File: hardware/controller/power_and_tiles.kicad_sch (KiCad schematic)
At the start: 27 parts, among them U1 XDJK-0051-025, U2 EA8212HT6R, U3 MT3406

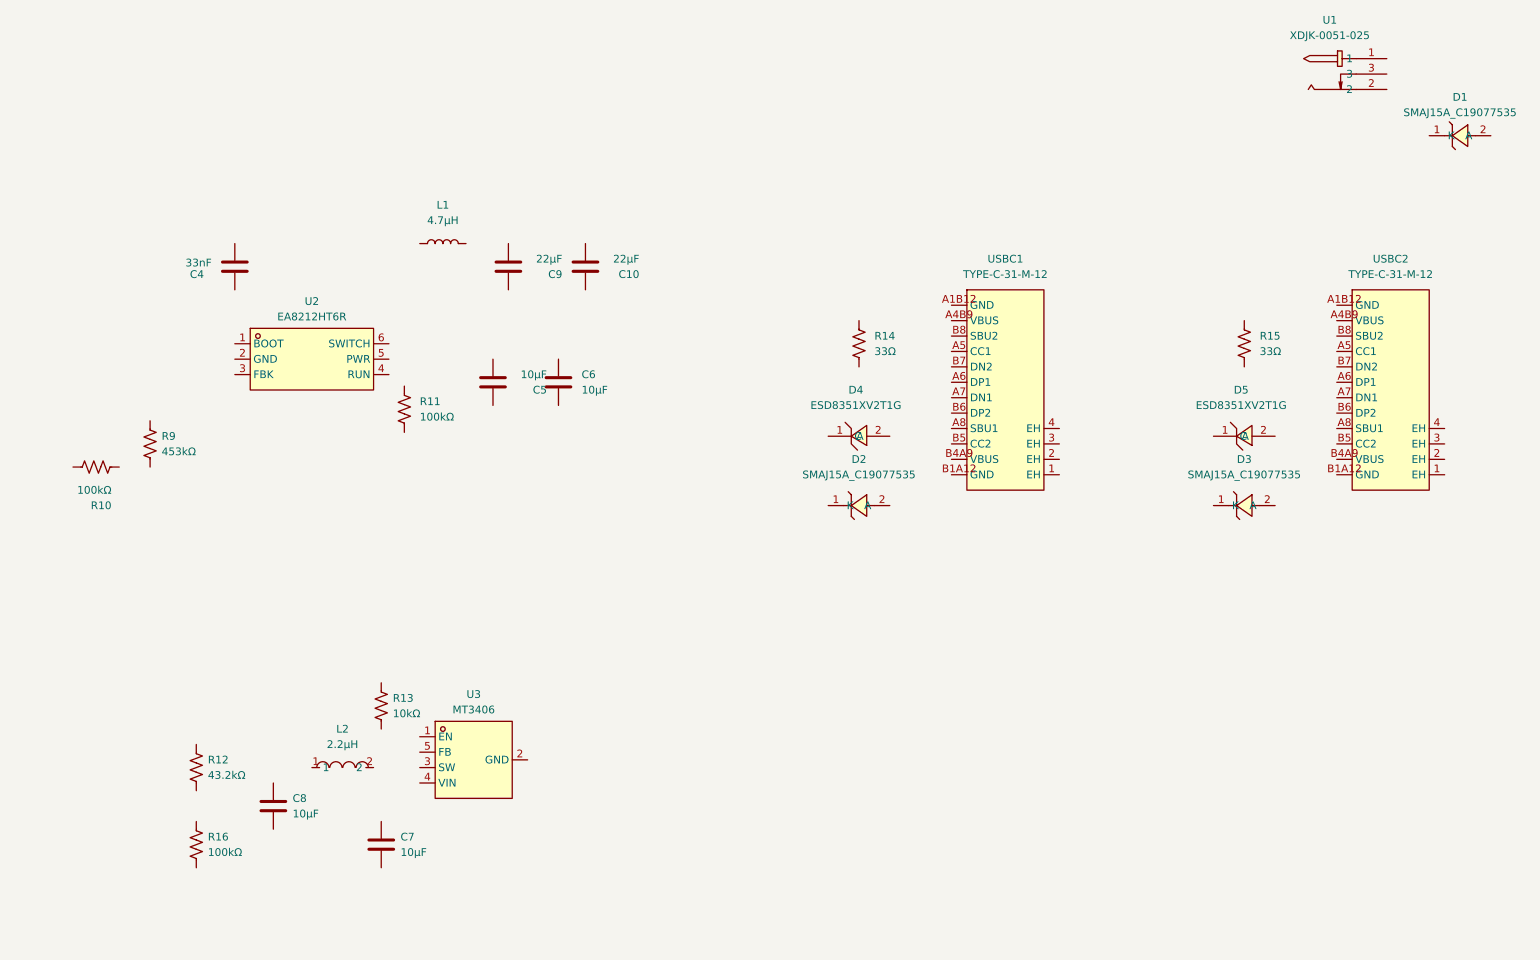
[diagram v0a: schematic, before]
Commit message: hooking up parts in the schematic
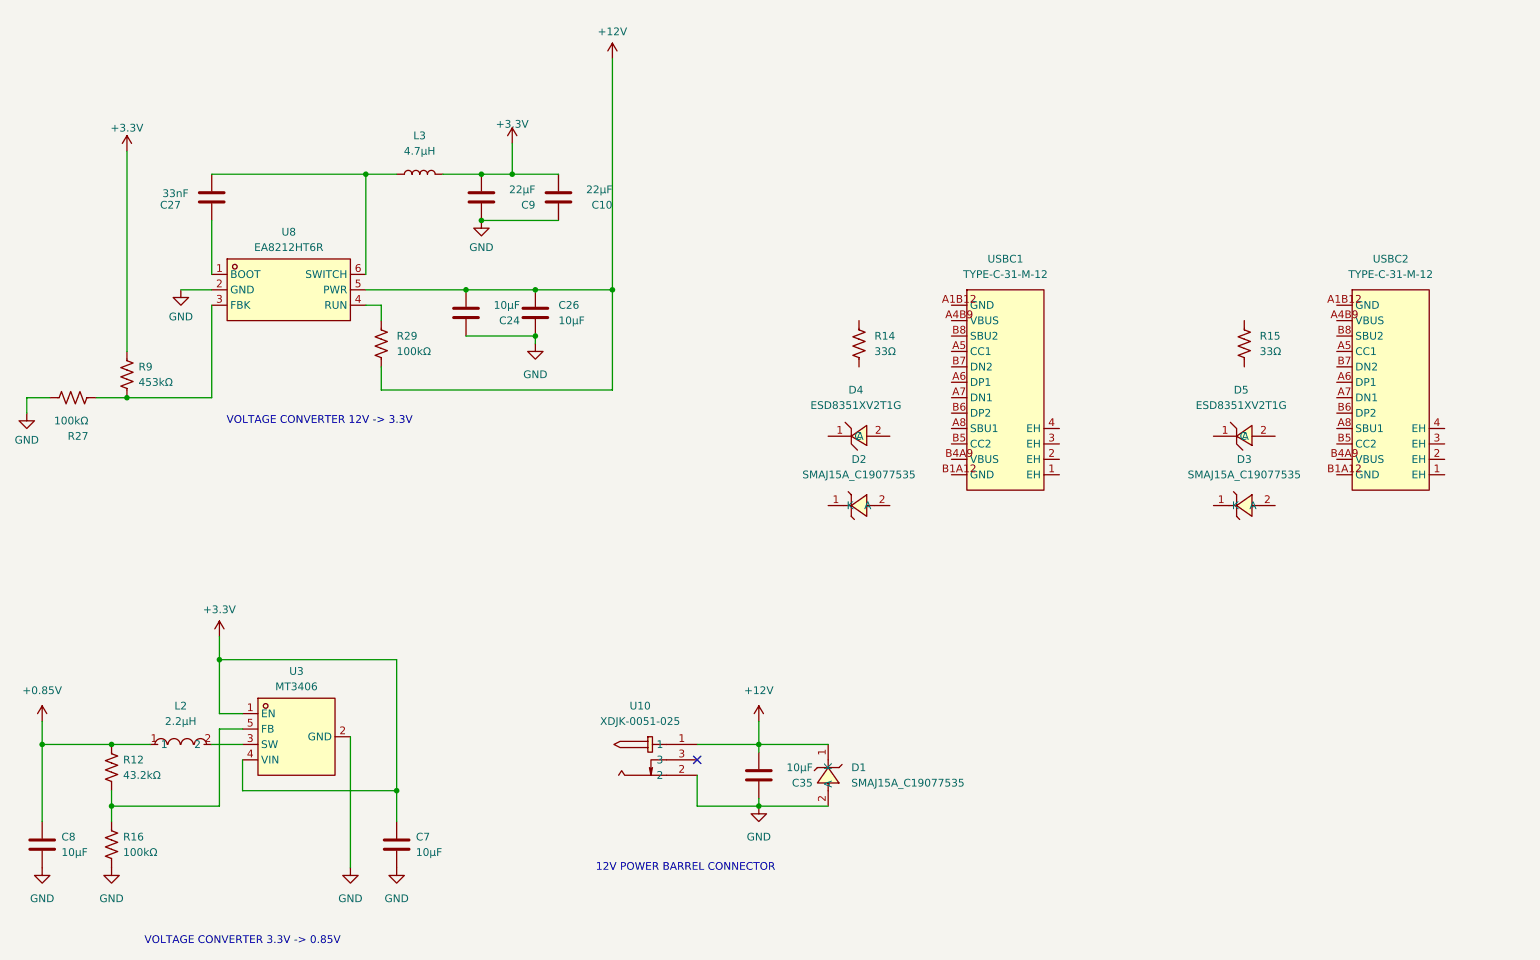
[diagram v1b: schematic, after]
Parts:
- removed C4: 33nF, Capacitor_SMD:C_0402_1005Metric, symbol Device:C
- removed C5, C6: 10µF, Capacitor_SMD:C_0603_1608Metric, symbol Device:C
- removed L1: 4.7µH, Inductor_SMD:L_Changjiang_FNR4030S, symbol Device:L
- removed R10, R11: 100kΩ, Resistor_SMD:R_0402_1005Metric, symbol Device:R_US
- removed R13: 10kΩ, Resistor_SMD:R_0402_1005Metric, symbol Device:R_US
- removed U1: XDJK-0051-025, easyeda2kicad:DC-IN-TH_XDJK-0051-025, symbol easyeda2kicad:XDJK-0051-025
- removed U2: EA8212HT6R, easyeda2kicad:SOT-23-6_L2.9-W1.6-P0.95-LS2.8-BR, symbol easyeda2kicad:EA8212HT6R
- added C24, C26, C35: 10µF, Capacitor_SMD:C_0603_1608Metric, symbol Device:C
- added C27: 33nF, Capacitor_SMD:C_0402_1005Metric, symbol Device:C
- added L3: 4.7µH, Inductor_SMD:L_Changjiang_FNR4030S, symbol Device:L
- added R27, R29: 100kΩ, Resistor_SMD:R_0402_1005Metric, symbol Device:R_US
- added U10: XDJK-0051-025, easyeda2kicad:DC-IN-TH_XDJK-0051-025, symbol easyeda2kicad:XDJK-0051-025
- added U8: EA8212HT6R, easyeda2kicad:SOT-23-6_L2.9-W1.6-P0.95-LS2.8-BR, symbol easyeda2kicad:EA8212HT6R
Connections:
- net +3.3V: now reaches C10.1
- net +3.3V: now also C7.1, C9.1, R9.2, U3.1 (EN), U3.4 (VIN), L3.2
- net GND: now reaches C10.2
- net GND: now also C7.2, C8.2, C9.2, D1.2 (A), R16.2, U3.2 (GND), C24.2, C26.2, C35.2, R27.2, U10.2, U8.2 (GND)
- net +0.85V: now reaches L2.1
- net +0.85V: now also C8.1, R12.1
- net at L2.2: now also U3.3 (SW)
- net at R16.1: now also R12.2, U3.5 (FB)
- net at R9.1: now also R27.1, U8.3 (FBK)
- net +12V: now reaches D1.1 (K)
- net +12V: now also C24.1, C26.1, C35.1, R29.2, U10.1, U8.5 (PWR)
- new net: C27.1, U8.1 (BOOT)
- new net: C27.2, L3.1, U8.6 (SWITCH)
- new net: R29.1, U8.4 (RUN)
- no-connect marks 0 -> 1
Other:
- note added: "12V POWER BARREL CONNECTOR"
- note added: "VOLTAGE CONVERTER 12V -> 3.3V"
- note added: "VOLTAGE CONVERTER 3.3V -> 0.85V"
- moved on the sheet: C10, C7, C8, C9, D1, L2, R12, R16, R9, U3
